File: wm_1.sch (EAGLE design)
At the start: 22 parts, among them T1 MMBT3904, T2 BT138-V, X1 22-23-2031

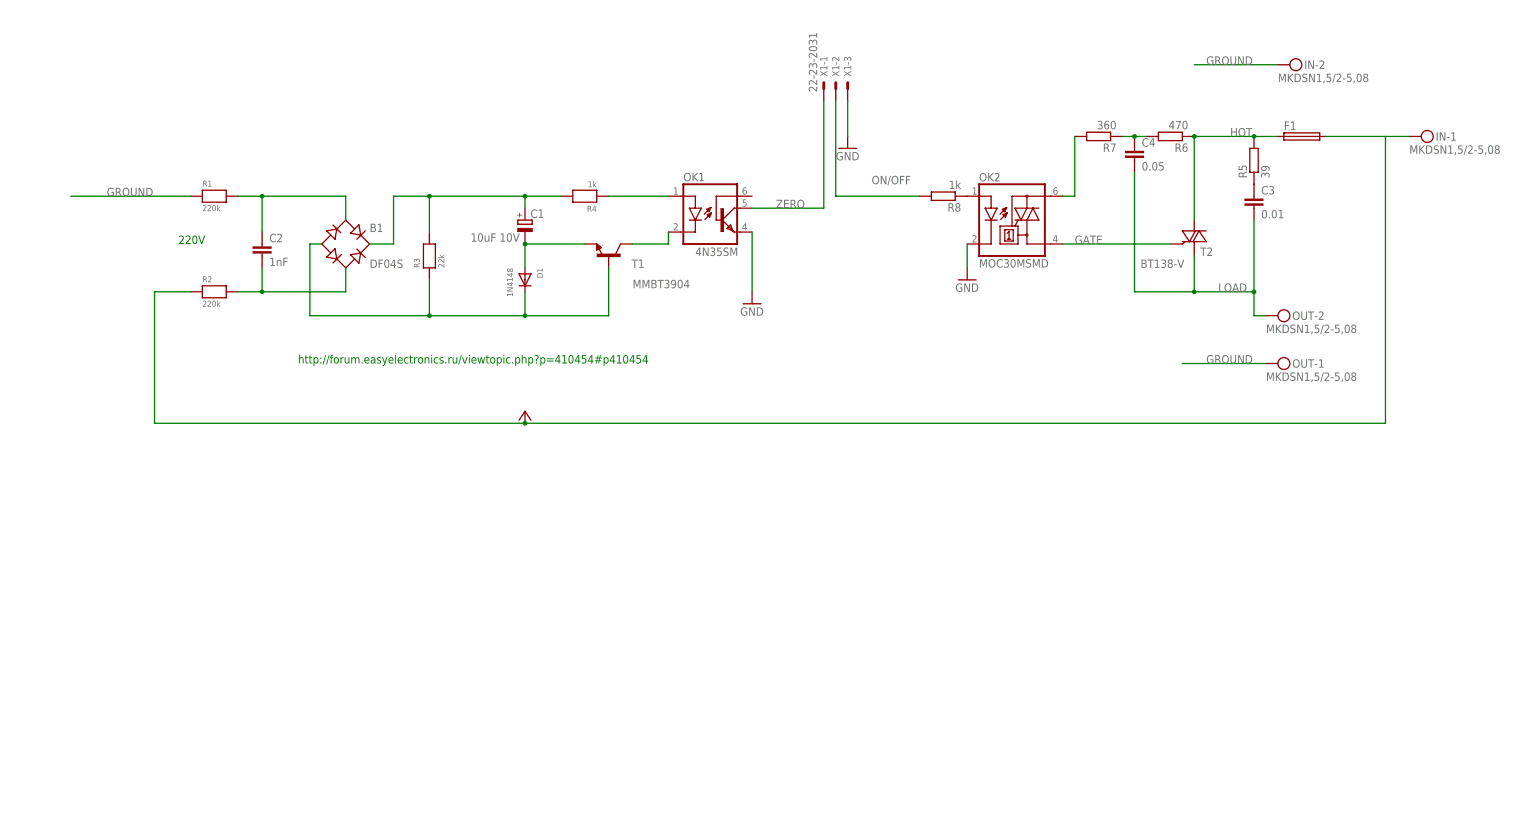
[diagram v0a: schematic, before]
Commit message: v2.1
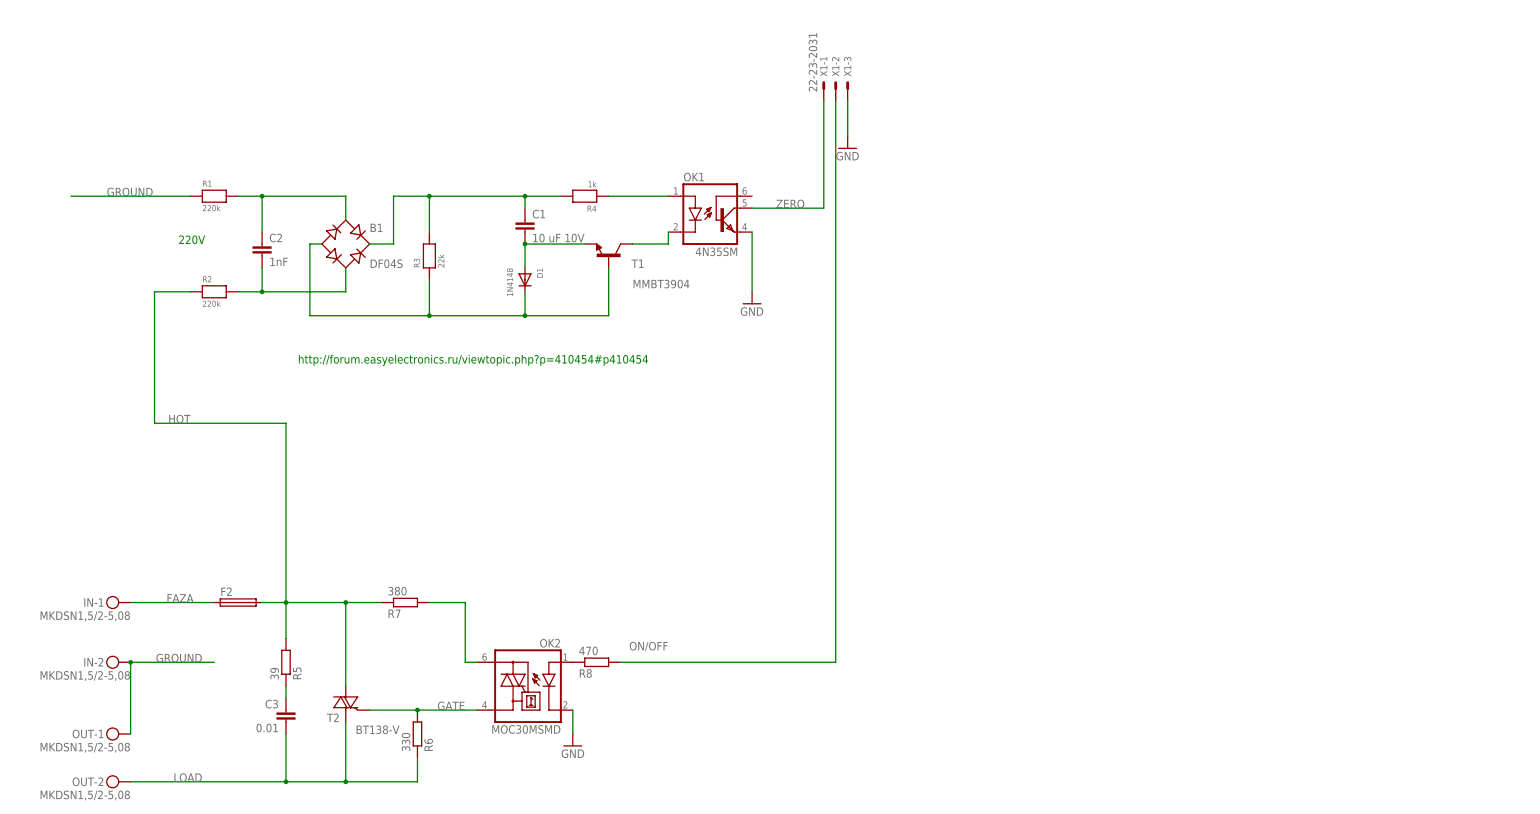
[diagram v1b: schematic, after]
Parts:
- removed C4: 0.05, rcl:C-EUC1206
- removed F1: (no value), fuse:GSH15
- added F2: (no value), fuse:SH22,5A
- C1: value 10uF 10V -> 10 uF 10V; device rcl:CPOL-EU140CLH-1010 -> rcl:C-EUC1206
- C2: device rcl:C-EUC0805 -> rcl:C-EUC1206
- R6: value 470 -> 330
- R7: value 360 -> 380
- R8: value 1k -> 470
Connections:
- removed net N$8: C4.1, R6.2, R7.1
- removed net N$9: F1.2, IN-1.KL, R2.1
- new net FAZA: F2.1, IN-1.KL
- net GATE: now also R6.2
- net HOT: now also F2.2, R2.1, R7.1; no longer F1.1, R6.1
- net LOAD: now also R6.1; no longer C4.2
- net N$3: now also C1.2; no longer C1.-
- net N$5: now also C1.1; no longer C1.+
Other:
- moved on the sheet: C3, IN-1, IN-2, OK2, OUT-1, OUT-2, R5, R6, R7, R8, T2
